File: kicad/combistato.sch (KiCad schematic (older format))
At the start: 7 parts

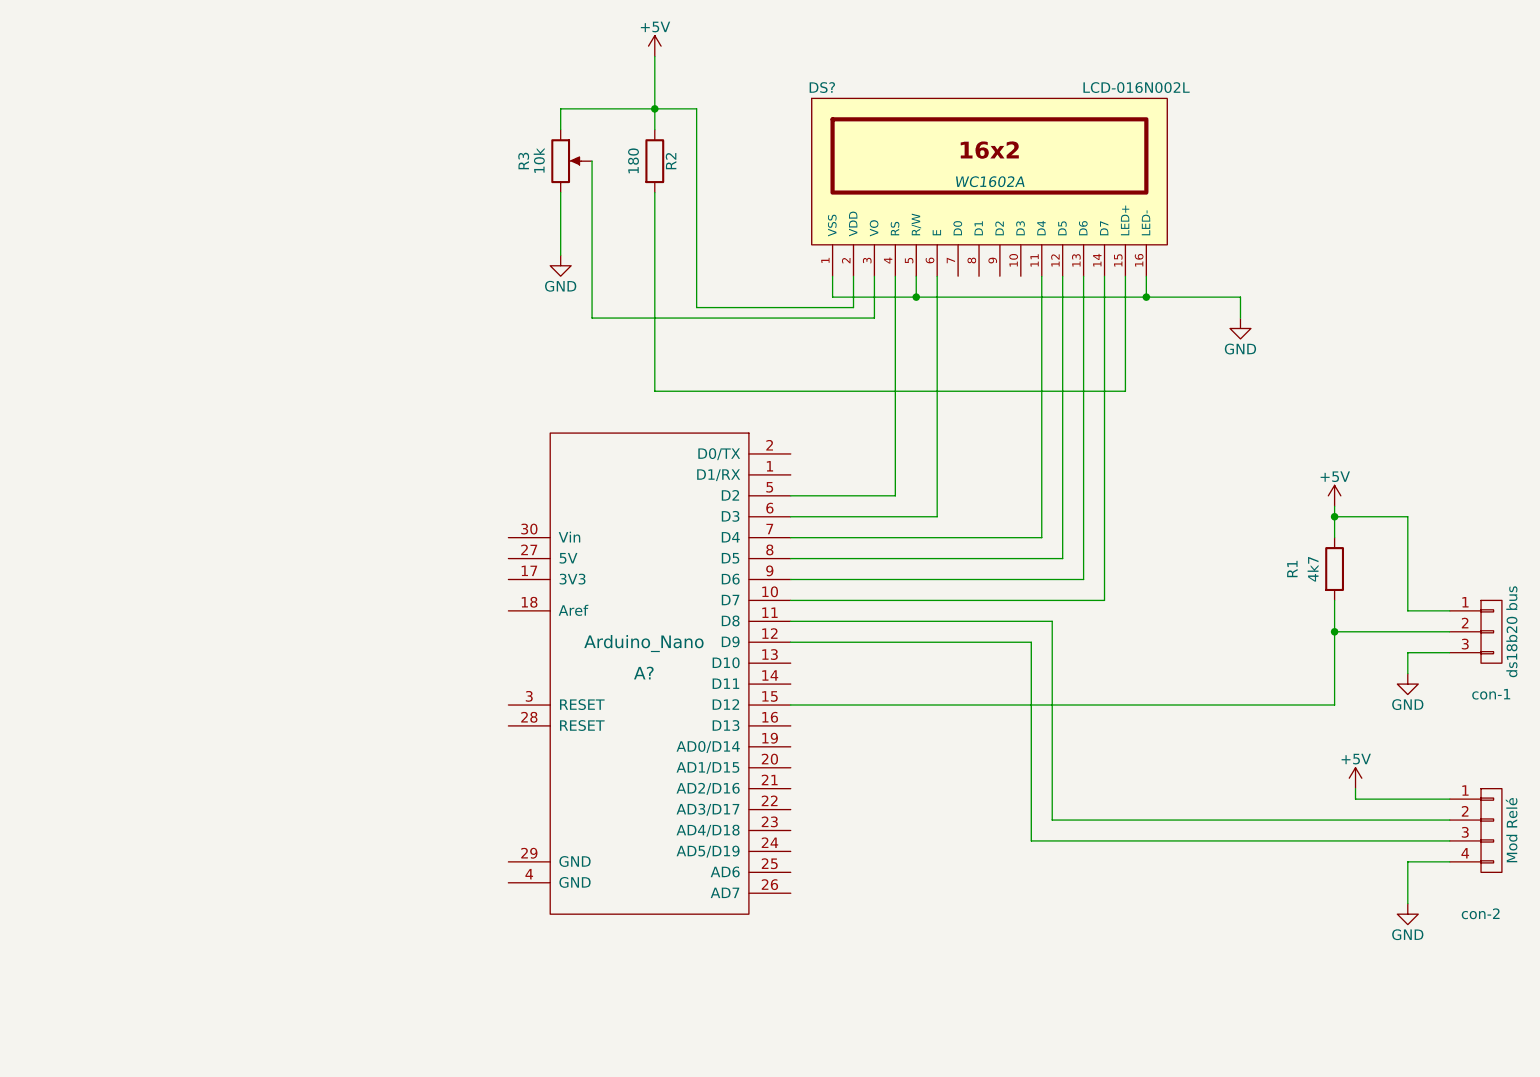
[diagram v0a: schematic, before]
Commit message: trabajo en pcb, circuitos, etc
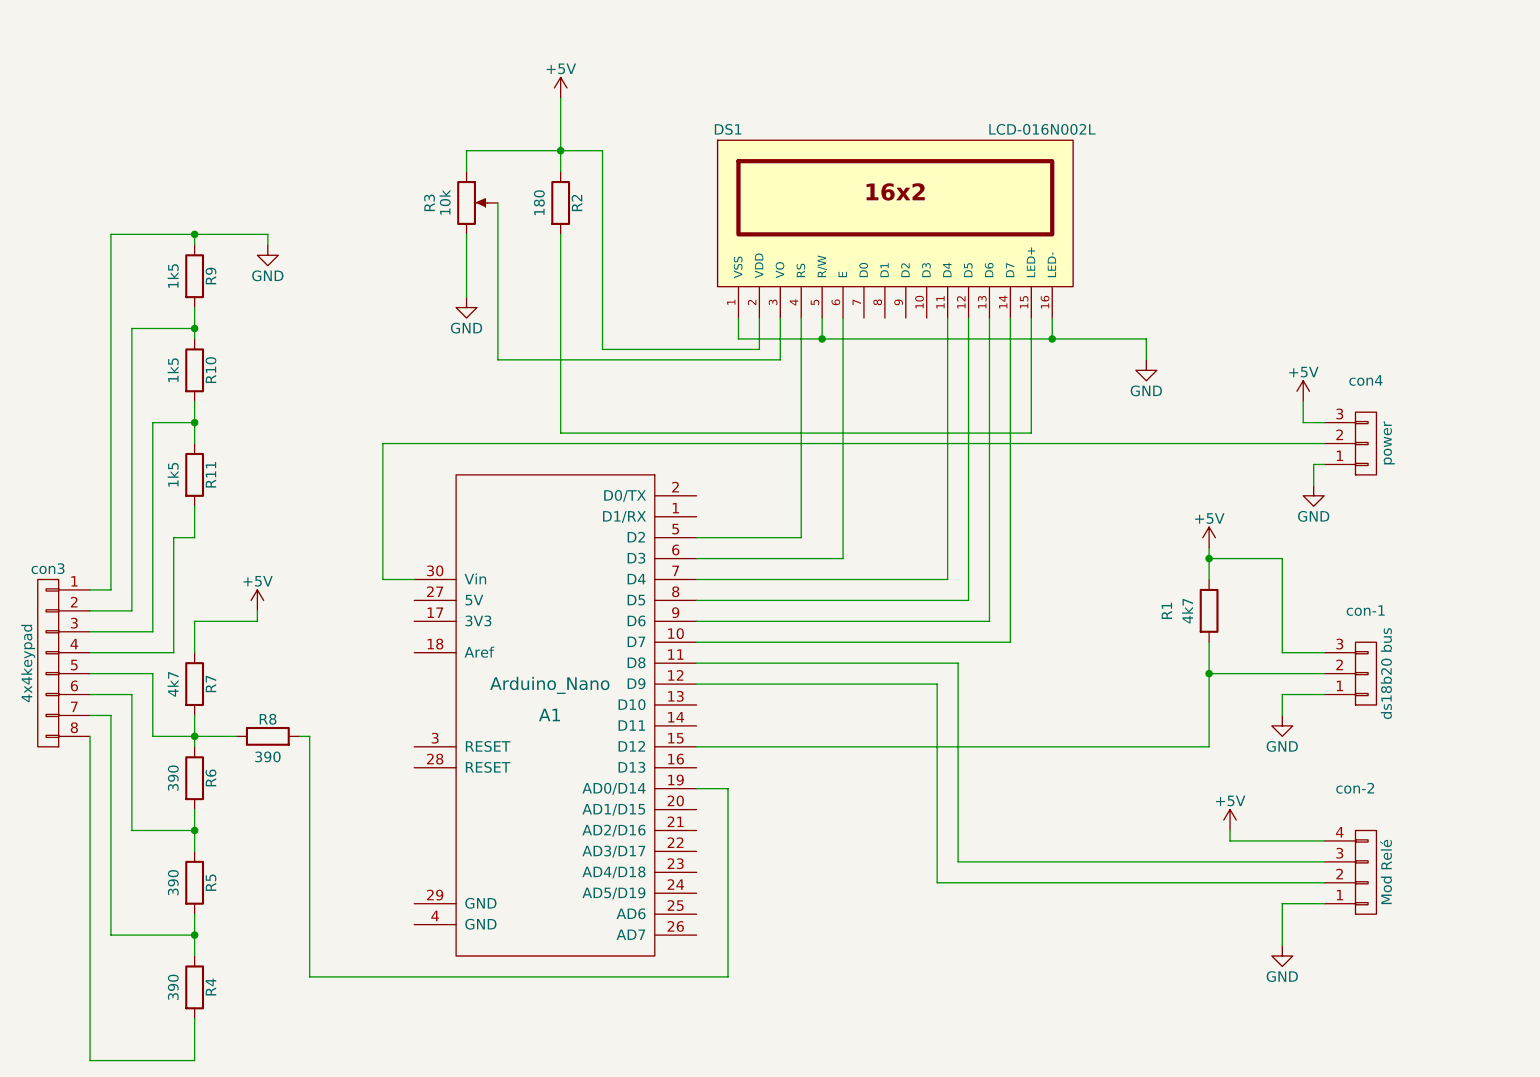
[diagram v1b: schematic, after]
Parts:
- removed A?: Arduino_Nano, symbol Arduino_Nano
- added A1: Arduino_Nano, Arduino Nano:arduino_nano, symbol Arduino_Nano
- added R10, R11, R9: 1k5, Resistores convencionales:R_Axial_DIN0411_L9.9mm_D3.6mm_P12.70mm_Horizontal, symbol R
- added R4, R5, R6, R8: 390, Resistores convencionales:R_Axial_DIN0411_L9.9mm_D3.6mm_P12.70mm_Horizontal, symbol R
- added R7: 4k7, Resistores convencionales:R_Axial_DIN0411_L9.9mm_D3.6mm_P12.70mm_Horizontal, symbol R
- added con3: 4x4keypad, Pin_Headers:Pin_Header_Angled_1x08, symbol CONN_01X08
- added con4: power, Pin_Headers:Pin_Header_Angled_1x03, symbol CONN_01X03
- DS1: renamed from DS?; footprint WC1602A -> LCD 1602:wc1602
- R1, R2: footprint (none) -> Resistores convencionales:R_Axial_DIN0411_L9.9mm_D3.6mm_P12.70mm_Horizontal
- R3: footprint (none) -> Potentiometers:Potentiometer_Bourns_3339H_Angular_ScrewUp
- con-1: footprint (none) -> Pin_Headers:Pin_Header_Angled_1x03
- con-2: footprint (none) -> Pin_Headers:Pin_Header_Angled_1x04
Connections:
- net +5V: now also con-1.3 (P3), con-2.4 (P4), R7.1, con4.3 (P3); no longer con-1.1 (P1), con-2.1 (P1)
- net GND: now also con-1.1 (P1), con-2.1 (P1), R9.1, con3.1 (P1), con4.1 (P1); no longer con-1.3 (P3), con-2.4 (P4)
- net at DS1.14 (D7): now also A1.10 (D7)
- net at con-2.2 (P2): now also A1.12 (D9)
- net at con-2.3 (P3): now also A1.11 (D8)
- net at R1.2, con-1.2 (P2): now also A1.15 (D12)
- net at DS1.4 (RS): now also A1.5 (D2)
- net at DS1.6 (E): now also A1.6 (D3)
- net at DS1.11 (D4): now also A1.7 (D4)
- net at DS1.12 (D5): now also A1.8 (D5)
- net at DS1.13 (D6): now also A1.9 (D6)
- new net: R10.1, R9.2, con3.2 (P2)
- new net: R10.2, R11.1, con3.3 (P3)
- new net: R11.2, con3.4 (P4)
- new net: R6.1, R7.2, R8.1, con3.5 (P5)
- new net: R5.1, R6.2, con3.6 (P6)
- new net: R4.1, R5.2, con3.7 (P7)
- new net: R4.2, con3.8 (P8)
- new net: A1.19 (AD0/D14), R8.2
- new net: A1.30 (Vin), con4.2 (P2)
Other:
- moved on the sheet: DS1, R1, R2, R3, con-1, con-2
